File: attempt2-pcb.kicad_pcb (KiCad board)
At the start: 2 copper layers, 328.6 x 95.3 mm, 175 parts, among them J1 Conn_01x04, K1 keyboard_parts_KEYSW, K10 keyboard_parts_KEYSW, K11 keyboard_parts_KEYSW, K12 keyboard_parts_KEYSW, K13 keyboard_parts_KEYSW, K14 keyboard_parts_KEYSW, K15 keyboard_parts_KEYSW, K16 keyboard_parts_KEYSW, K17 keyboard_parts_KEYSW, K18 keyboard_parts_KEYSW, K19 keyboard_parts_KEYSW, K2 keyboard_parts_KEYSW, K20 keyboard_parts_KEYSW, K21 keyboard_parts_KEYSW, K22 keyboard_parts_KEYSW, K23 keyboard_parts_KEYSW, K24 keyboard_parts_KEYSW, K25 keyboard_parts_KEYSW, K26 keyboard_parts_KEYSW, K27 keyboard_parts_KEYSW, K28 keyboard_parts_KEYSW, K29 keyboard_parts_KEYSW, K3 keyboard_parts_KEYSW, K30 keyboard_parts_KEYSW, K31 keyboard_parts_KEYSW, K32 keyboard_parts_KEYSW, K33 keyboard_parts_KEYSW, K34 keyboard_parts_KEYSW, K35 keyboard_parts_KEYSW, K36 keyboard_parts_KEYSW, K37 keyboard_parts_KEYSW, K38 keyboard_parts_KEYSW, K39 keyboard_parts_KEYSW, K4 keyboard_parts_KEYSW, K40 keyboard_parts_KEYSW, K41 keyboard_parts_KEYSW, K42 keyboard_parts_KEYSW, K43 keyboard_parts_KEYSW, K44 keyboard_parts_KEYSW, K45 keyboard_parts_KEYSW, K46 keyboard_parts_KEYSW, K47 keyboard_parts_KEYSW, K48 keyboard_parts_KEYSW, K49 keyboard_parts_KEYSW, K5 keyboard_parts_KEYSW, K50 keyboard_parts_KEYSW, K51 keyboard_parts_KEYSW, K52 keyboard_parts_KEYSW, K53 keyboard_parts_KEYSW, K54 keyboard_parts_KEYSW, K55 keyboard_parts_KEYSW, K56 keyboard_parts_KEYSW, K57 keyboard_parts_KEYSW, K58 keyboard_parts_KEYSW, K59 keyboard_parts_KEYSW, K6 keyboard_parts_KEYSW, K60 keyboard_parts_KEYSW, K61 keyboard_parts_KEYSW, K62 keyboard_parts_KEYSW, K63 keyboard_parts_KEYSW, K64 keyboard_parts_KEYSW, K65 keyboard_parts_KEYSW, K66 keyboard_parts_KEYSW, K67 keyboard_parts_KEYSW, K68 keyboard_parts_KEYSW, K69 keyboard_parts_KEYSW, K7 keyboard_parts_KEYSW, K70 keyboard_parts_KEYSW, K71 keyboard_parts_KEYSW, K72 keyboard_parts_KEYSW, K73 keyboard_parts_KEYSW, K74 keyboard_parts_KEYSW, K75 keyboard_parts_KEYSW, K76 keyboard_parts_KEYSW, K77 keyboard_parts_KEYSW, K78 keyboard_parts_KEYSW, K79 keyboard_parts_KEYSW, K8 keyboard_parts_KEYSW, K80 keyboard_parts_KEYSW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

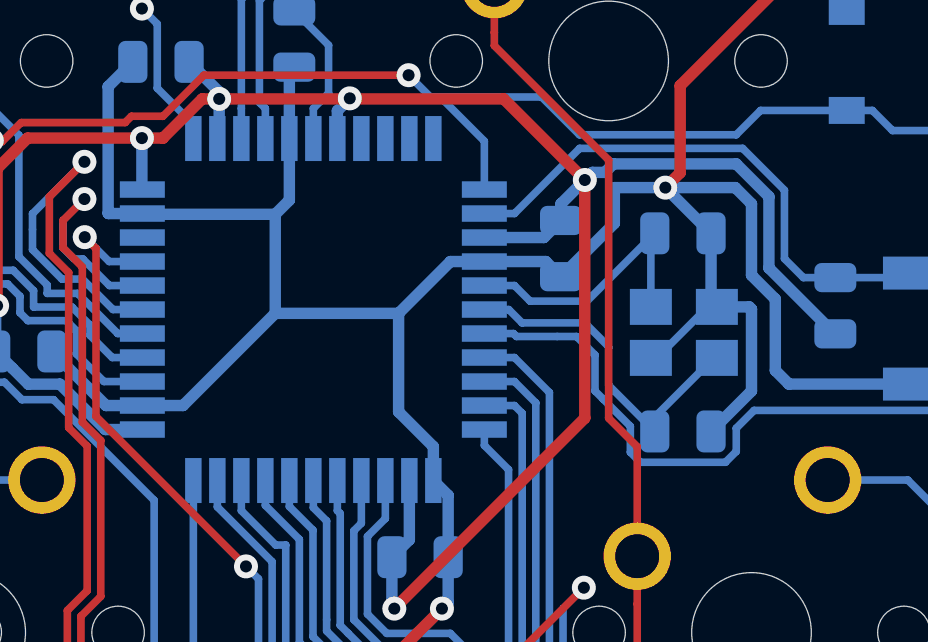
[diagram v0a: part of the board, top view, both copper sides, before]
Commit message: Fill Zones
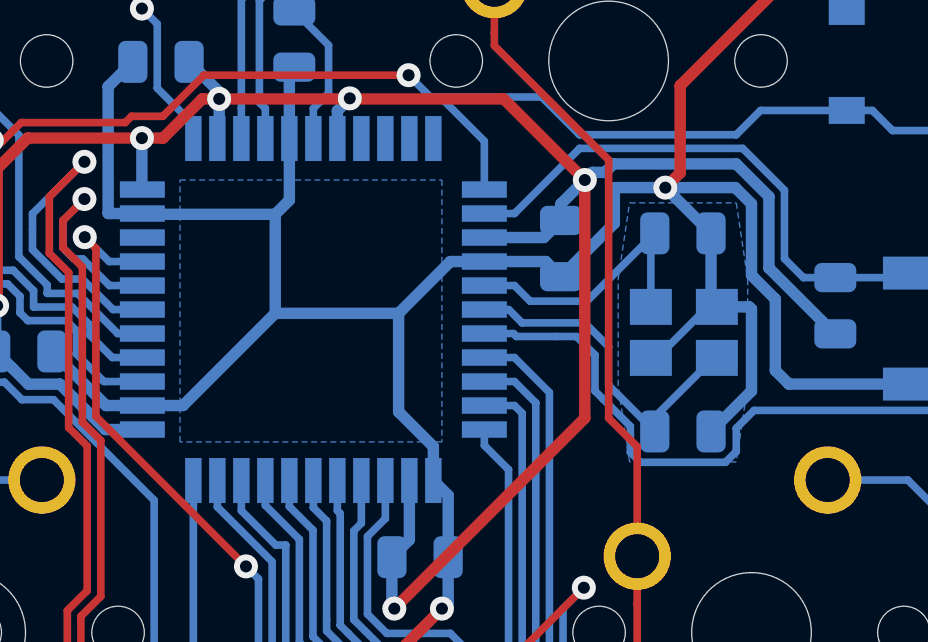
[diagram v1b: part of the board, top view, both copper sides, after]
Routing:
- added copper zone on B.Cu, net GND
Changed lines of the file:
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@@
   (segment (start 98.87 89.105) (end 98.425 89.55) (width 0.254) (layer B.Cu) (net 109))
   (segment (start 98.87 83.043) (end 98.87 89.105) (width 0.254) (layer B.Cu) (net 109))
+  (zone (net 1) (net_name GND) (layer B.Cu) (hatch edge 0.508)
+    (connect_pads (clearance 0.508))
+    (min_thickness 0.254)
+    (fill yes (arc_segments 32) (thermal_gap 0.508) (thermal_bridge_width 0.508))
+    (polygon
+      (pts
+        (xy 98.425 73.025) (xy 107.15625 73.025) (xy 107.15625 81.75625) (xy 98.425 81.75625)
+      )
+    )
+  )
+  (zone (net 1) (net_name GND) (layer B.Cu) (hatch edge 0.508)
+    (connect_pads (clearance 0.508))
+    (min_thickness 0.254)
+    (fill yes (arc_segments 32) (thermal_gap 0.508) (thermal_bridge_width 0.508))
+    (polygon
+      (pts
+        (xy 113.411 73.787) (xy 116.967 73.787) (xy 117.348 76.327) (xy 117.348 79.883) (xy 116.967 82.423)
+        (xy 113.411 82.423) (xy 113.03 79.883) (xy 113.03 76.327)
+      )
+    )
+  )
 )
